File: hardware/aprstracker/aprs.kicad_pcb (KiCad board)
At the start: 2 copper layers, 102 x 38 mm, 122 parts, among them IC1 ATMEGA8-AI, J1 SMA, J2 SMA, P1 CONN_6, P3 CONN_2, Q1 MMBT5551, Q2 MMBT5551, Q3 BCX54, Q4 BFR93A, Q5 BFR93A, Q6 BFG135, Q7 MMBT5551, U1 LM7001, U2 EB-3531, U3 78L33, U4 78L05, X1 CRYSTAL, X2 CRYSTAL

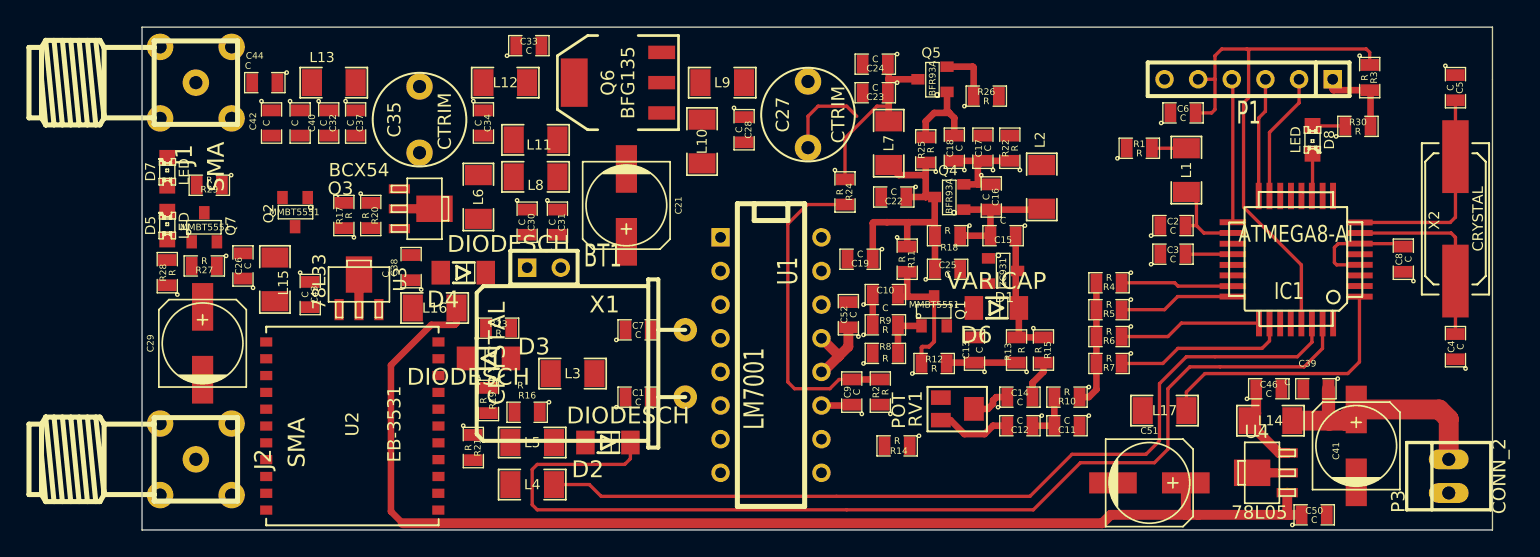
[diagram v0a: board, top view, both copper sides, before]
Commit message: [HW] route pcb
Signed-off-by: Angel Hitov <angelhitov@gmail.com>
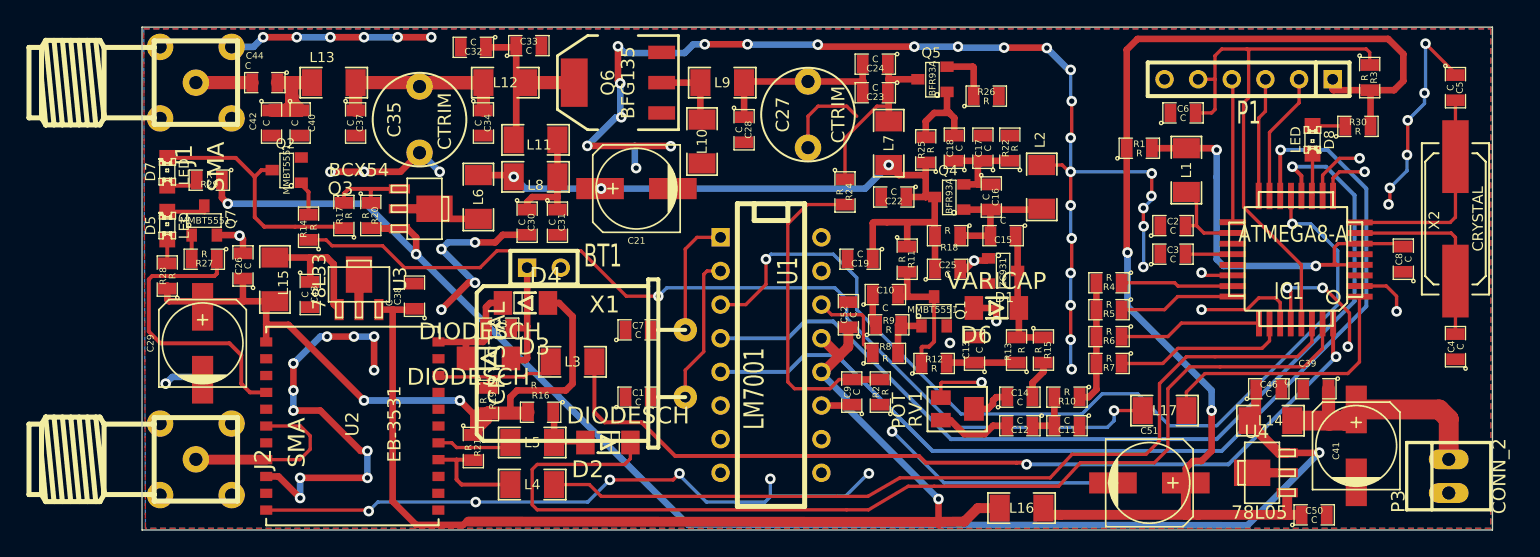
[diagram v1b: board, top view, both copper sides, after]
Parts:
- moved R14 47.4 mm to (108.8, 96.9), turned to 90 degrees
- moved L16 46.8 mm to (162.7, 118.1)
- moved C32 12.3 mm to (121.3, 83.3), turned to 180 degrees
- moved D4 5.23 mm to (125.2, 102.6), turned to 0 degrees
- moved Q2 3.24 mm to (107.2, 92.6), turned to 90 degrees
- moved C38 2.17 mm to (116.8, 102.1)
- moved C21 1.48 mm to (133.6, 94.0), turned to 180 degrees
- moved R16 1.02 mm to (126.4, 110.9)
- moved L3 0.89 mm to (128.8, 107.1)
- moved R27 0.51 mm to (101.0, 99.3)
- moved Q7 0.51 mm to (101.0, 96.4)
- moved R29 0.38 mm to (101.3, 93.3)
- moved R28 0.25 mm to (98.2, 100.6)
- moved R9 0.25 mm to (152.7, 104.3)
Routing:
- net GND: track 6.69 -> 266.8 mm, vias 0 -> 70
- net VDD: track 7.79 -> 113.1 mm, vias 0 -> 3
- net +5V: track 6.26 -> 86.3 mm, vias 0 -> 1
- net DATA: track 0.00 -> 76.9 mm, vias 0 -> 1
- net CL: track 0.00 -> 72.5 mm, vias 0 -> 1
- net N-0000029: track 0.00 -> 72.2 mm, vias 0 -> 2
- net CE: track 0.00 -> 71.7 mm, vias 0 -> 2
- net RF_PWR: track 0.00 -> 67.4 mm, vias 0 -> 2
- net 3V3: track 0.00 -> 57.9 mm, vias 0 -> 2
- net N-0000094: track 23.0 -> 56.3 mm, vias 0 -> 3
- net N-000002: track 0.00 -> 22.4 mm
- net N-0000044: track 11.1 -> 31.3 mm, vias 0 -> 2
- net N-0000091: track 0.00 -> 20.0 mm
- net N-0000064: track 0.00 -> 18.8 mm
- net N-0000067: track 0.00 -> 14.7 mm
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- added copper zone on B.Cu, net GND
- added copper zone on F.Cu, net GND
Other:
- rule via_min_drill: 0.508 -> 0.4
- rule via_min_size: 0.889 -> 0.8
